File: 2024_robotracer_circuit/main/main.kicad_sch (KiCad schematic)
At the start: 69 parts, among them J1 PH_6p, J10 PH_5p, J11 PH_6p, J13 PH_8p, J2 Conn_02x05_Odd_Even, J3 Conn_02x05_Odd_Even, J4 PA_2p, J5 PA_2p, J6 XT_2p, J7 HX_12p, J8 PH_4p, J9 PH_5p, SW1 TVGP01-G73BB, U1 STM32F405RGTx, U10 MTN2306AN3, U16 AE-BMX055, U17 MTN2306AN3, U2 SIT2001B, U22 SKRHAAE010, U23 SS-22F32G5, U3 AM2837, U4 AM2837, U5 BP5293-33, U6 BP5293-50, U7 SSM6J808R, U8 MTN2306AN3

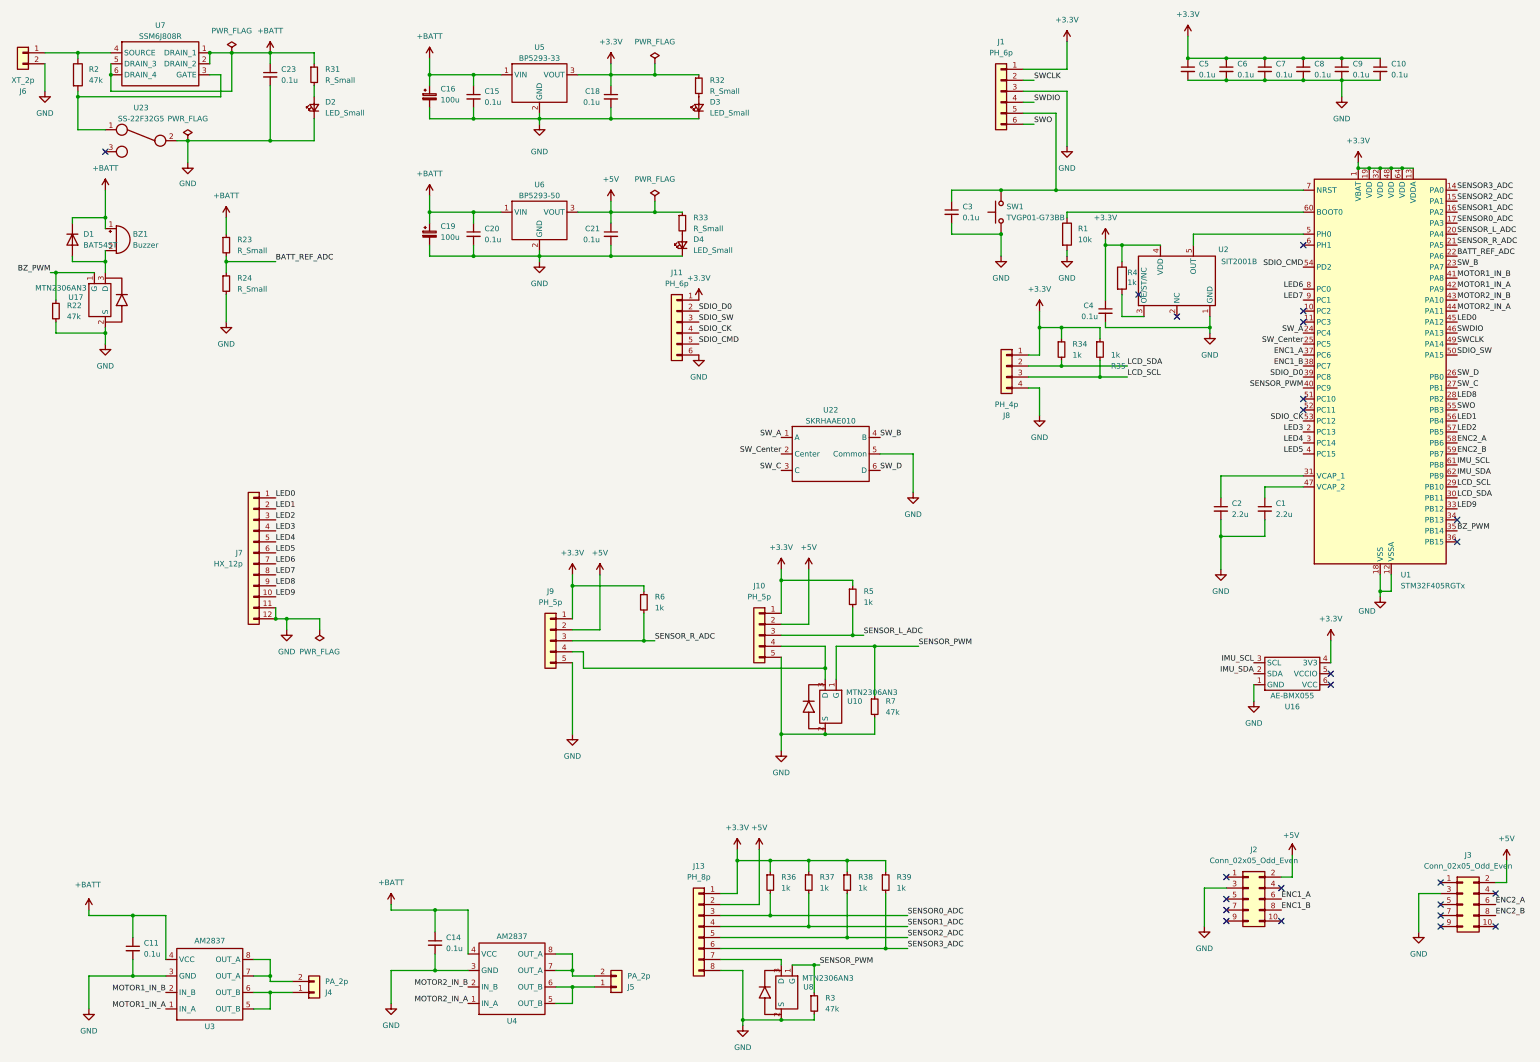
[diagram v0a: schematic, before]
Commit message: 修正
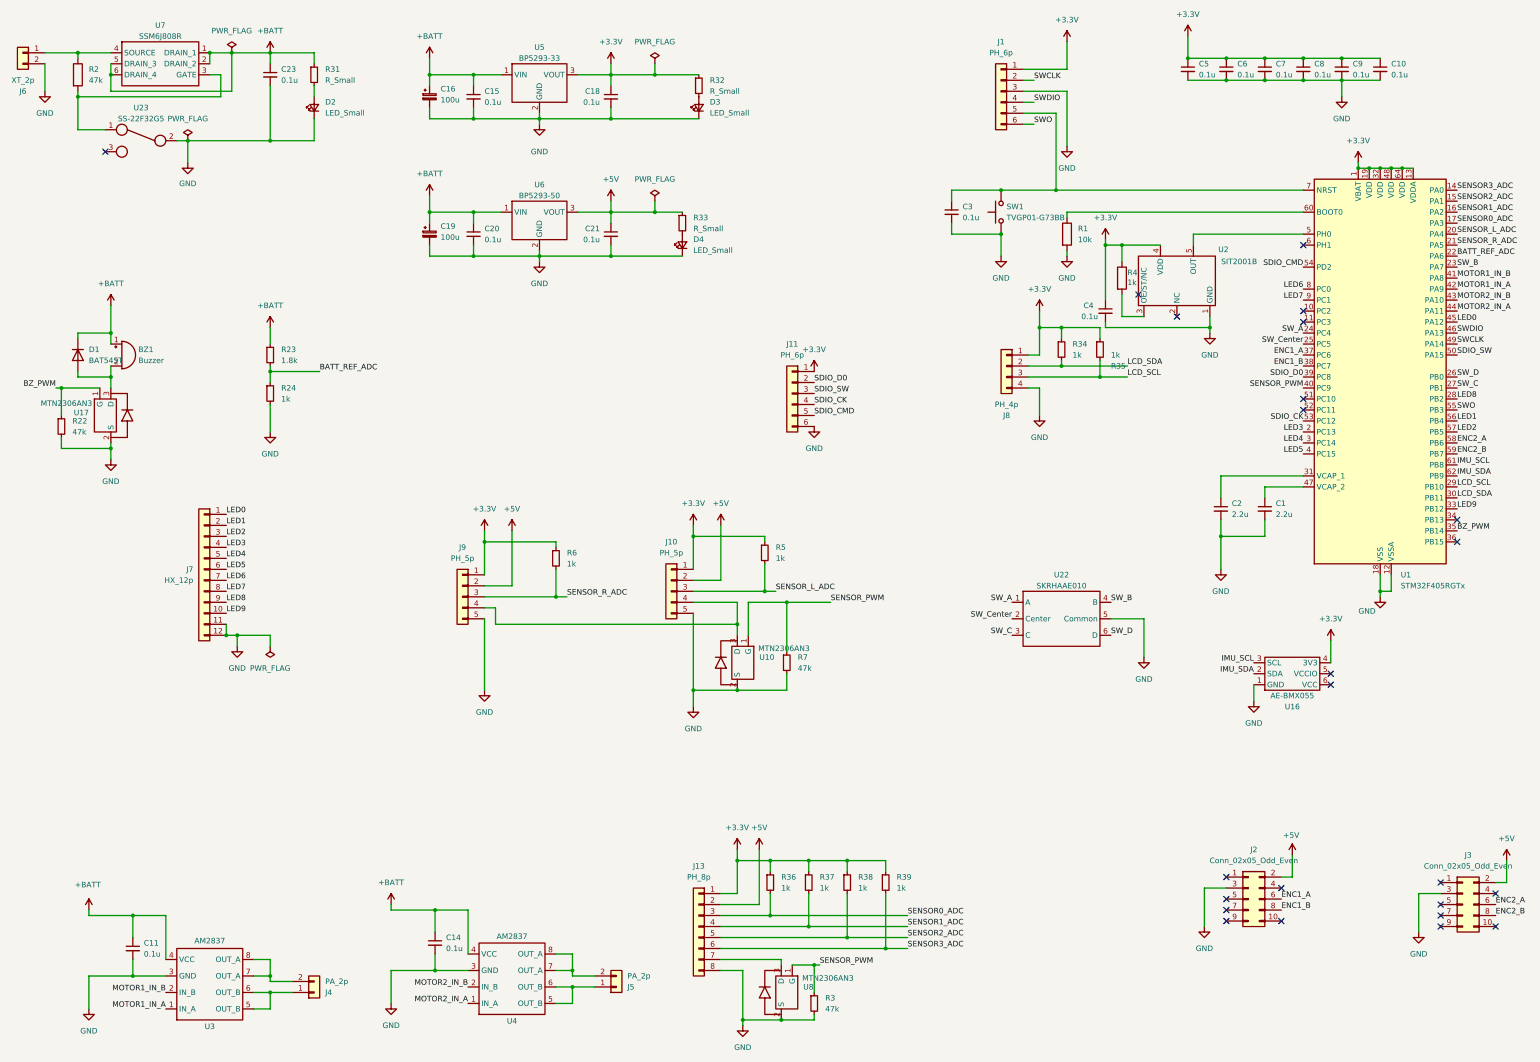
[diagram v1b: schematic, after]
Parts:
- R23: value R_Small -> 1.8k
- R24: value R_Small -> 1k
- U3, U4: footprint Package_SO:TSSOP-8_3x3mm_P0.65mm -> Package_SO:SOP-8_3.9x4.9mm_P1.27mm
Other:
- moved on the sheet: BZ1, D1, J10, J11, J7, J9, R22, R23, R24, R5, R6, R7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
